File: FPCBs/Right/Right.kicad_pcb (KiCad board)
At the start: 2 copper layers, 53 x 77.1 mm, 20 parts, among them J1 PCB, SW1 Mode Dial, SW2 ON/OFF, SW3 Focus+Shutter, SW4 Focus+Shutter, U1 SG-105, U2 SG-105

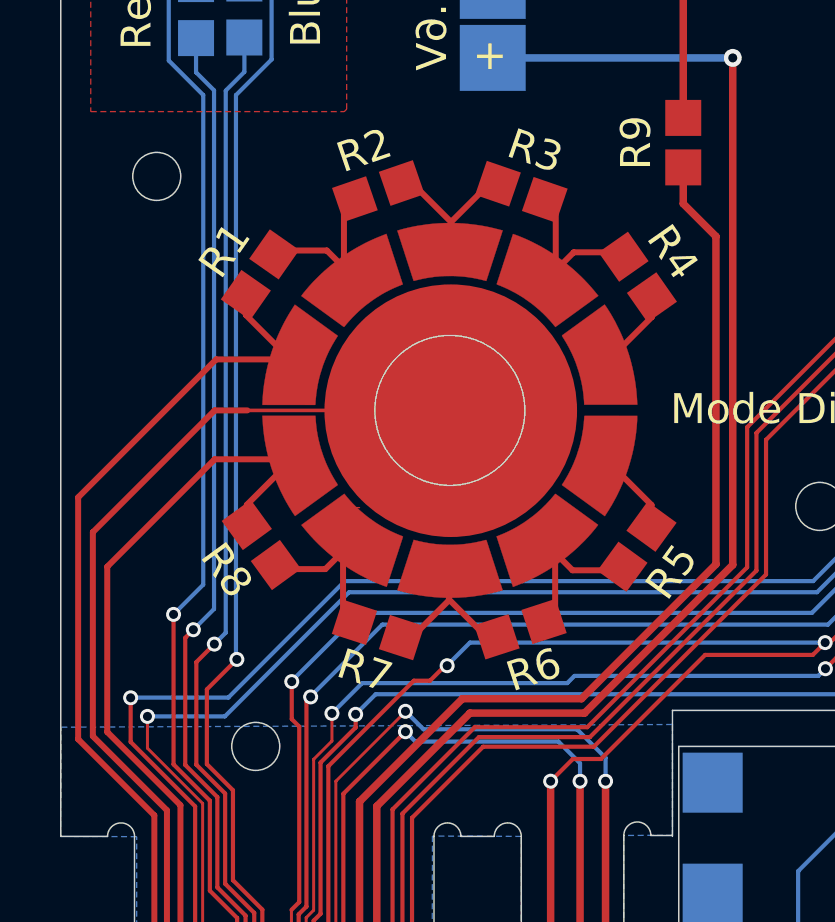
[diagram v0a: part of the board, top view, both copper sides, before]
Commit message: Fix left fpcb
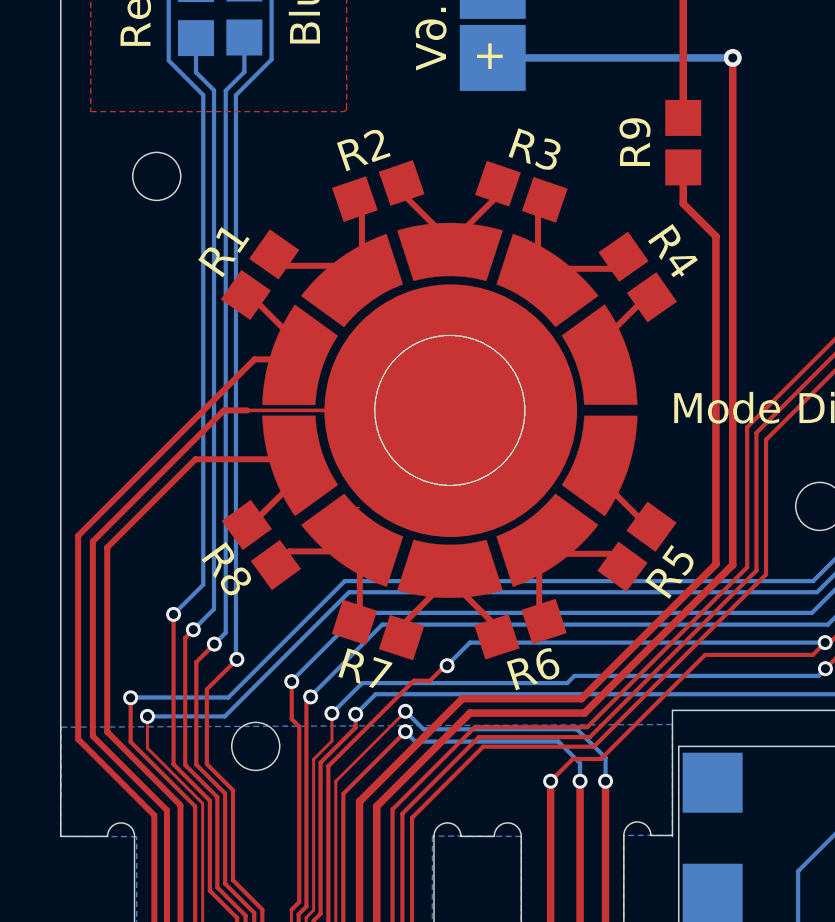
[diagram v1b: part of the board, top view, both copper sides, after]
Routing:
- net Net-(R2-Pad2): track 5.17 -> 4.30 mm
- net Net-(J1-Pin_1): track 73.3 -> 72.5 mm
